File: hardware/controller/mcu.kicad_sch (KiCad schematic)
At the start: 20 parts, among them J12 USB_C_Receptacle_USB2.0_14P, J5 Screw_Terminal_01x02, J6 Screw_Terminal_01x02, U1 ESP32-C3-MINI-1, U6 TPS1H200AQDGNRQ1

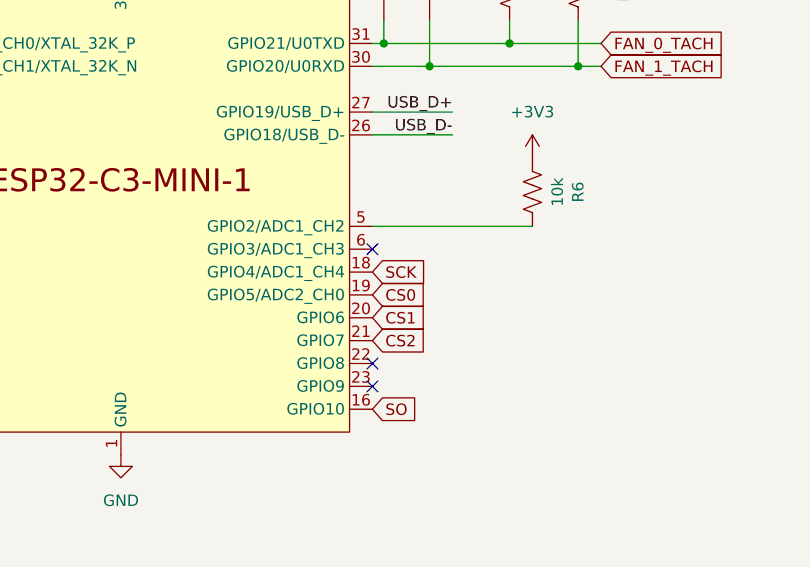
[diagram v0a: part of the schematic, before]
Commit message: First stab at board routing
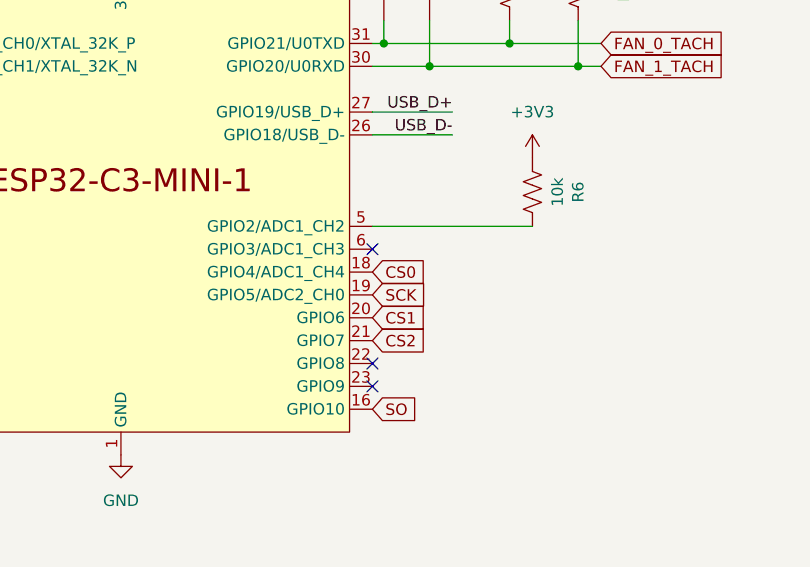
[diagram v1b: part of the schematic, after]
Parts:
- TP4, TP5: footprint TestPoint:TestPoint_Pad_D2.0mm -> TestPoint:TestPoint_THTPad_2.0x2.0mm_Drill1.0mm
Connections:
- net CS0: now also U1.18 (GPIO4/ADC1_CH4); no longer U1.19 (GPIO5/ADC2_CH0)
- net SCK: now also U1.19 (GPIO5/ADC2_CH0); no longer U1.18 (GPIO4/ADC1_CH4)
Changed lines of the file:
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@@
 	(global_label "SCK"
 		(shape input)
-		(at 173.99 100.33 0)
+		(at 173.99 102.87 0)
 		(fields_autoplaced yes)
 		(effects
@@
 		)
 		(property "Intersheetrefs" "${INTERSHEET_REFS}"
-			(at 180.7247 100.33 0)
+			(at 180.7247 102.87 0)
 			(effects
 				(font
@@
 	(global_label "CS0"
 		(shape input)
-		(at 173.99 102.87 0)
+		(at 173.99 100.33 0)
 		(fields_autoplaced yes)
 		(effects
@@
 		)
 		(property "Intersheetrefs" "${INTERSHEET_REFS}"
-			(at 180.6642 102.87 0)
+			(at 180.6642 100.33 0)
 			(effects
 				(font
@@
 			)
 		)
-		(property "Footprint" "TestPoint:TestPoint_Pad_D2.0mm"
+		(property "Footprint" "TestPoint:TestPoint_THTPad_2.0x2.0mm_Drill1.0mm"
 			(at 180.34 72.39 0)
 			(effects
@@
 			)
 		)
-		(property "Footprint" "TestPoint:TestPoint_Pad_D2.0mm"
+		(property "Footprint" "TestPoint:TestPoint_THTPad_2.0x2.0mm_Drill1.0mm"
 			(at 185.42 72.39 0)
 			(effects
